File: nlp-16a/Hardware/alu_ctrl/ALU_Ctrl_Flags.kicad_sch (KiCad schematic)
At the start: 18 parts, among them U1 CD74HC00, U10 CD74HC00, U11 CD74HC00, U12 CD74HC00, U13 CD74HC00, U14 CD74HC00, U15 CD74HC00, U16 CD74HC00, U17 CD74HC00, U18 CD74HC00, U2 CD74HC00, U3 CD74HC00, U4 CD74HC00, U5 CD74HC00, U6 CD74HC00, U7 CD74HC00, U8 CD74HC00, U9 CD74HC00

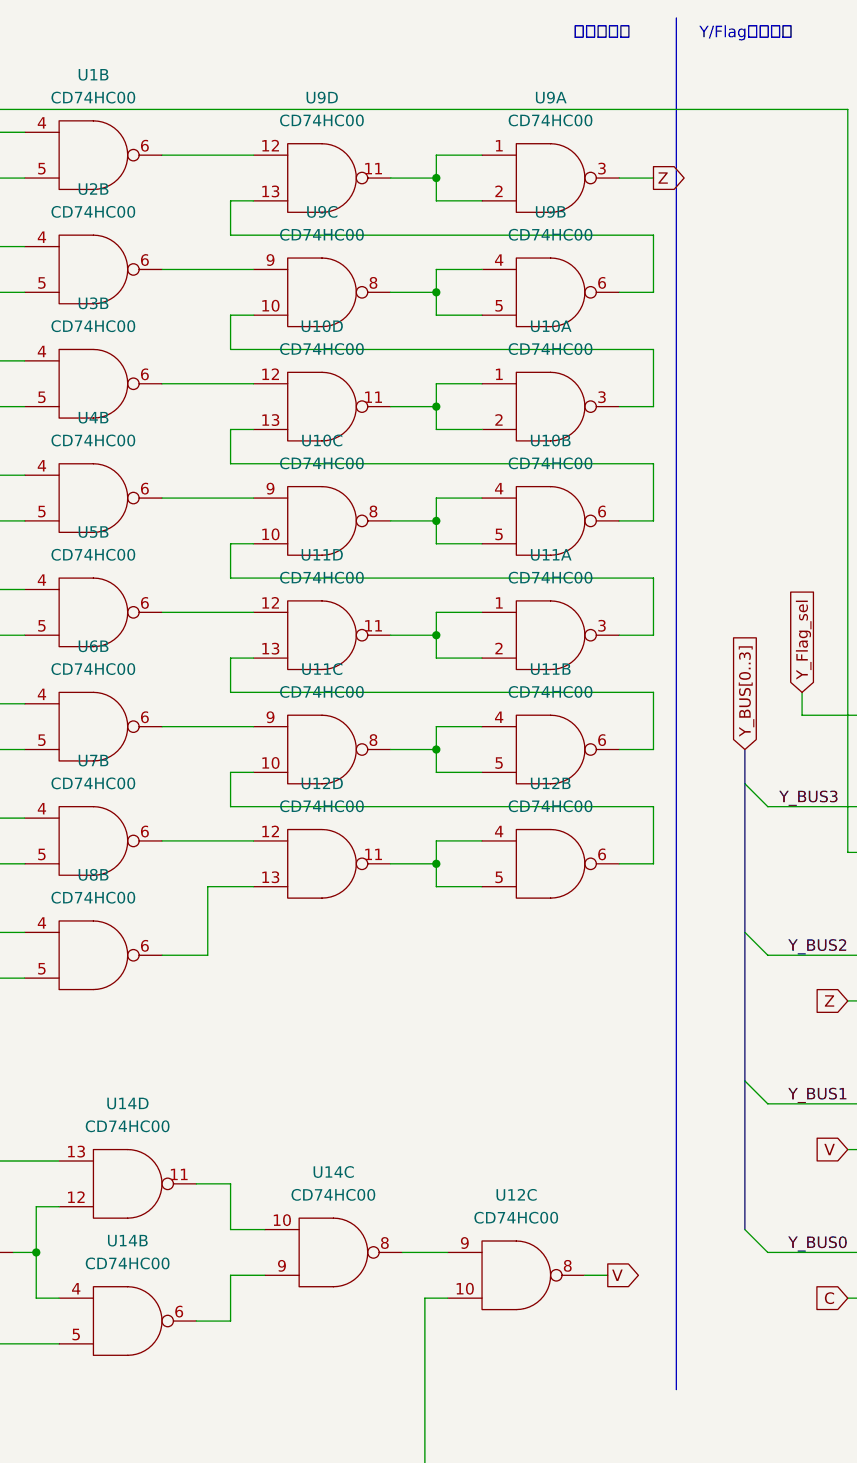
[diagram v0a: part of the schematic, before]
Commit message: 基板の途中経過
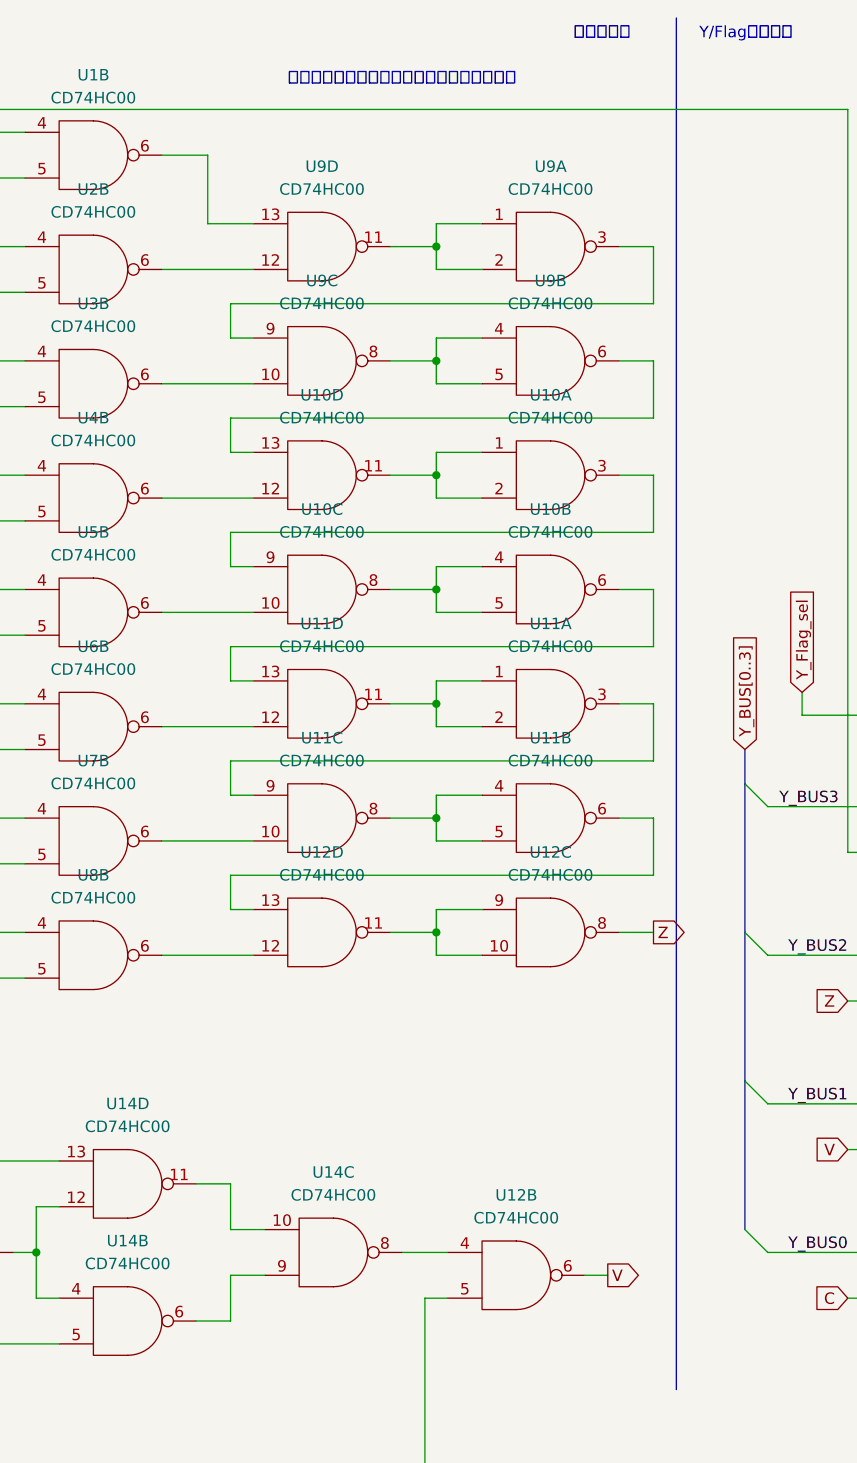
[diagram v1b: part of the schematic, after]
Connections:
- net V: now also U12.6; no longer U12.8
- net Z: now also U12.8; no longer U9.3
- net at U9.12: now also U2.6; no longer U1.6
- net at U9.13: now also U1.6; no longer U9.6
- net at U10.12: now also U4.6; no longer U3.6
- net at U10.13: now also U9.6; no longer U10.6
- net at U11.10: now also U7.6; no longer U12.6
- net at U11.9: now also U11.3; no longer U6.6
- net at U15.8: now also U12.5; no longer U12.10
- net at U14.8: now also U12.4; no longer U12.9
- net at U12.12: now also U8.6; no longer U7.6
- net at U10.9: now also U10.3; no longer U4.6
- net at U10.10: now also U5.6; no longer U11.3
- net at U12.13: now also U11.6; no longer U8.6
- net at U11.12: now also U6.6; no longer U5.6
- net at U11.13: now also U10.6; no longer U11.6
- net at U9.10: now also U3.6; no longer U10.3
- net at U9.9: now also U9.3; no longer U2.6
- new net: U12.10, U12.11, U12.9
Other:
- note added: "配線の容易さを優先し，最速の接続ではない"
- moved on the sheet: U10A, U10B, U10C, U10D, U11A, U11B, U11C, U11D, U12C, U12D, U9A, U9B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

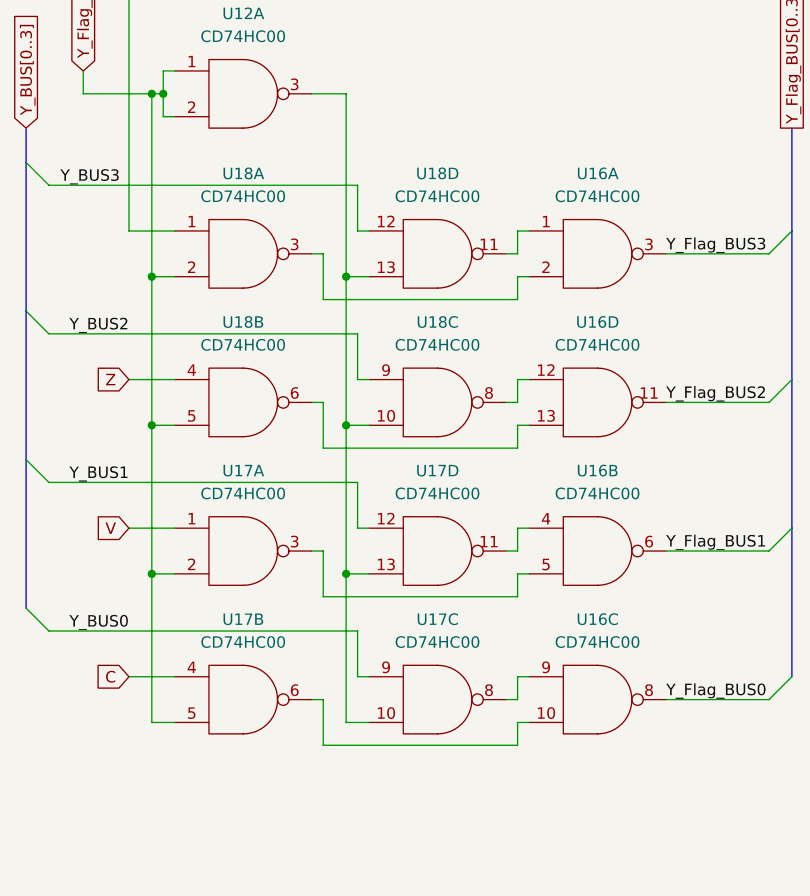
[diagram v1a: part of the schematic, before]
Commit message: デコーダ周りの配線が通った!
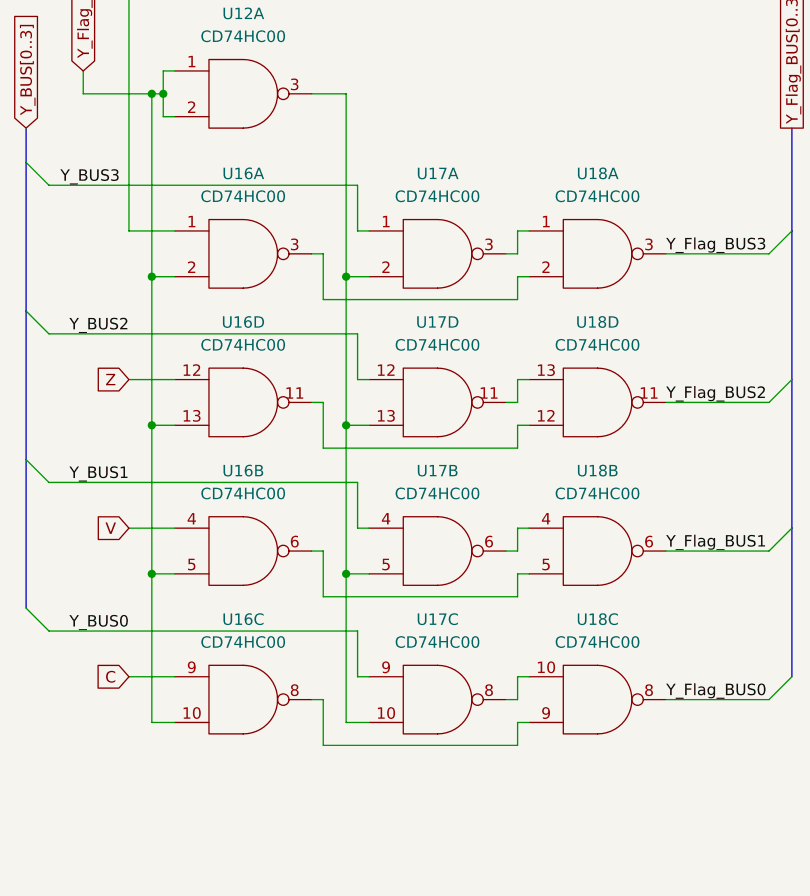
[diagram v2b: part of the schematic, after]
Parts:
- renumbered U18 to U16, U17 to U16, U18 to U17, U16 to U18
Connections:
- net C: now also U16.9; no longer U16.4
- net V: now also U16.4; no longer U16.1
- net Y_BUS1: now also U17.4; no longer U17.12
- net Y_BUS2: now also U17.12; no longer U17.9
- net Y_BUS3: now also U17.1; no longer U17.12
- net Y_Flag_sel: now also U16.10, U16.13, U16.5; no longer U16.2, U16.5, U16.5
- net Z: now also U16.12; no longer U16.4
- net at U18.5: now also U16.6; no longer U16.3
- net at U18.12: now also U16.11; no longer U17.8
- net at U18.13: now also U17.11; no longer U16.6
- net at U18.10: now also U17.8; no longer U16.6
- net at U18.4: now also U17.6; no longer U17.11
- net at U18.1: now also U17.3; no longer U17.11
- net at U18.9: now also U16.8; no longer U17.8
- new net: U12.3, U17.10, U17.13, U17.2, U17.5
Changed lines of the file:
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@@
   (symbol (lib_id "CD74HCxx:CD74HC00") (at 222.25 107.95 0) (unit 1)
     (in_bom yes) (on_board yes) (fields_autoplaced)
-    (property "Reference" "U18" (id 0) (at 222.25 99.06 0))
+    (property "Reference" "U16" (id 0) (at 222.25 99.06 0))
     (property "Value" "CD74HC00" (id 1) (at 222.25 101.6 0))
     (property "Footprint" "Package_DIP:DIP-14_W7.62mm" (id 2) (at 217.17 107.95 0)
@@
     (pin "13")
   )
-  (symbol (lib_id "CD74HCxx:CD74HC00") (at 222.25 140.97 0) (unit 1)
-    (in_bom yes) (on_board yes) (fields_autoplaced)
-    (property "Reference" "U17" (id 0) (at 222.25 132.08 0))
+  (symbol (lib_id "CD74HCxx:CD74HC00") (at 222.25 140.97 0) (unit 2)
+    (in_bom yes) (on_board yes) (fields_autoplaced)
+    (property "Reference" "U16" (id 0) (at 222.25 132.08 0))
     (property "Value" "CD74HC00" (id 1) (at 222.25 134.62 0))
     (property "Footprint" "Package_DIP:DIP-14_W7.62mm" (id 2) (at 217.17 140.97 0)
@@
     (pin "13")
   )
-  (symbol (lib_id "CD74HCxx:CD74HC00") (at 243.84 124.46 0) (unit 3)
-    (in_bom yes) (on_board yes) (fields_autoplaced)
-    (property "Reference" "U18" (id 0) (at 243.84 115.57 0))
+  (symbol (lib_id "CD74HCxx:CD74HC00") (at 243.84 124.46 0) (unit 4)
+    (in_bom yes) (on_board yes) (fields_autoplaced)
+    (property "Reference" "U17" (id 0) (at 243.84 115.57 0))
     (property "Value" "CD74HC00" (id 1) (at 243.84 118.11 0))
     (property "Footprint" "Package_DIP:DIP-14_W7.62mm" (id 2) (at 238.76 124.46 0)
@@
     (pin "13")
   )
-  (symbol (lib_id "CD74HCxx:CD74HC00") (at 261.62 124.46 0) (unit 4)
-    (in_bom yes) (on_board yes) (fields_autoplaced)
-    (property "Reference" "U16" (id 0) (at 261.62 115.57 0))
+  (symbol (lib_id "CD74HCxx:CD74HC00") (at 261.62 124.46 0) (mirror x) (unit 4)
+    (in_bom yes) (on_board yes) (fields_autoplaced)
+    (property "Reference" "U18" (id 0) (at 261.62 115.57 0))
     (property "Value" "CD74HC00" (id 1) (at 261.62 118.11 0))
     (property "Footprint" "Package_DIP:DIP-14_W7.62mm" (id 2) (at 256.54 124.46 0)
@@
     (pin "13")
   )
-  (symbol (lib_id "CD74HCxx:CD74HC00") (at 222.25 157.48 0) (unit 2)
-    (in_bom yes) (on_board yes) (fields_autoplaced)
-    (property "Reference" "U17" (id 0) (at 222.25 148.59 0))
+  (symbol (lib_id "CD74HCxx:CD74HC00") (at 222.25 157.48 0) (unit 3)
+    (in_bom yes) (on_board yes) (fields_autoplaced)
+    (property "Reference" "U16" (id 0) (at 222.25 148.59 0))
     (property "Value" "CD74HC00" (id 1) (at 222.25 151.13 0))
     (property "Footprint" "Package_DIP:DIP-14_W7.62mm" (id 2) (at 217.17 157.48 0)
@@
     (pin "13")
   )
-  (symbol (lib_id "CD74HCxx:CD74HC00") (at 243.84 140.97 0) (unit 4)
+  (symbol (lib_id "CD74HCxx:CD74HC00") (at 243.84 140.97 0) (unit 2)
     (in_bom yes) (on_board yes) (fields_autoplaced)
     (property "Reference" "U17" (id 0) (at 243.84 132.08 0))
@@
     (pin "13")
   )
-  (symbol (lib_id "CD74HCxx:CD74HC00") (at 222.25 124.46 0) (unit 2)
-    (in_bom yes) (on_board yes) (fields_autoplaced)
-    (property "Reference" "U18" (id 0) (at 222.25 115.57 0))
+  (symbol (lib_id "CD74HCxx:CD74HC00") (at 222.25 124.46 0) (unit 4)
+    (in_bom yes) (on_board yes) (fields_autoplaced)
+    (property "Reference" "U16" (id 0) (at 222.25 115.57 0))
     (property "Value" "CD74HC00" (id 1) (at 222.25 118.11 0))
     (property "Footprint" "Package_DIP:DIP-14_W7.62mm" (id 2) (at 217.17 124.46 0)
@@
     (pin "13")
   )
-  (symbol (lib_id "CD74HCxx:CD74HC00") (at 243.84 107.95 0) (unit 4)
-    (in_bom yes) (on_board yes) (fields_autoplaced)
-    (property "Reference" "U18" (id 0) (at 243.84 99.06 0))
+  (symbol (lib_id "CD74HCxx:CD74HC00") (at 243.84 107.95 0) (unit 1)
+    (in_bom yes) (on_board yes) (fields_autoplaced)
+    (property "Reference" "U17" (id 0) (at 243.84 99.06 0))
     (property "Value" "CD74HC00" (id 1) (at 243.84 101.6 0))
     (property "Footprint" "Package_DIP:DIP-14_W7.62mm" (id 2) (at 238.76 107.95 0)
@@
     (pin "13")
   )
-  (symbol (lib_id "CD74HCxx:CD74HC00") (at 261.62 157.48 0) (unit 3)
-    (in_bom yes) (on_board yes) (fields_autoplaced)
-    (property "Reference" "U16" (id 0) (at 261.62 148.59 0))
+  (symbol (lib_id "CD74HCxx:CD74HC00") (at 261.62 157.48 0) (mirror x) (unit 3)
+    (in_bom yes) (on_board yes) (fields_autoplaced)
+    (property "Reference" "U18" (id 0) (at 261.62 148.59 0))
     (property "Value" "CD74HC00" (id 1) (at 261.62 151.13 0))
     (property "Footprint" "Package_DIP:DIP-14_W7.62mm" (id 2) (at 256.54 157.48 0)
@@
   (symbol (lib_id "CD74HCxx:CD74HC00") (at 261.62 140.97 0) (unit 2)
     (in_bom yes) (on_board yes) (fields_autoplaced)
-    (property "Reference" "U16" (id 0) (at 261.62 132.08 0))
+    (property "Reference" "U18" (id 0) (at 261.62 132.08 0))
     (property "Value" "CD74HC00" (id 1) (at 261.62 134.62 0))
     (property "Footprint" "Package_DIP:DIP-14_W7.62mm" (id 2) (at 256.54 140.97 0)
@@
   (symbol (lib_id "CD74HCxx:CD74HC00") (at 261.62 107.95 0) (unit 1)
     (in_bom yes) (on_board yes) (fields_autoplaced)
-    (property "Reference" "U16" (id 0) (at 261.62 99.06 0))
+    (property "Reference" "U18" (id 0) (at 261.62 99.06 0))
     (property "Value" "CD74HC00" (id 1) (at 261.62 101.6 0))
     (property "Footprint" "Package_DIP:DIP-14_W7.62mm" (id 2) (at 256.54 107.95 0)
